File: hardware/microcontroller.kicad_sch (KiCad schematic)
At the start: 12 parts, among them SW1 SW_DPST, U1 ATSAMD21G18A-M, Y1 Crystal

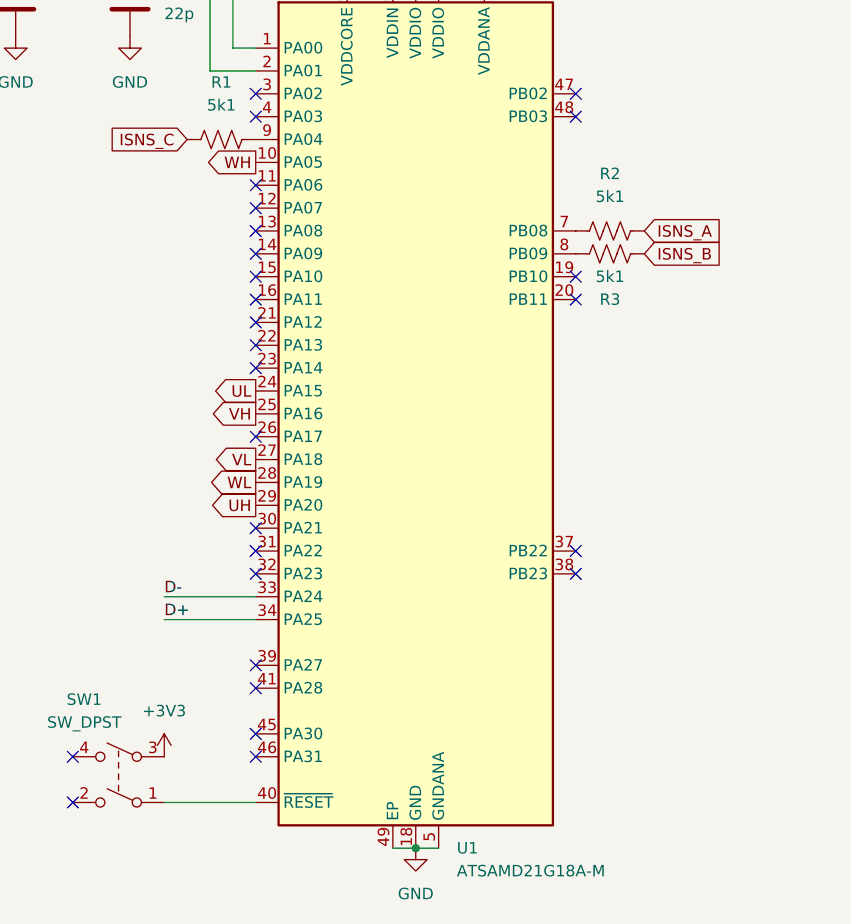
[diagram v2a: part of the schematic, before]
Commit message: Net changes, sense changes
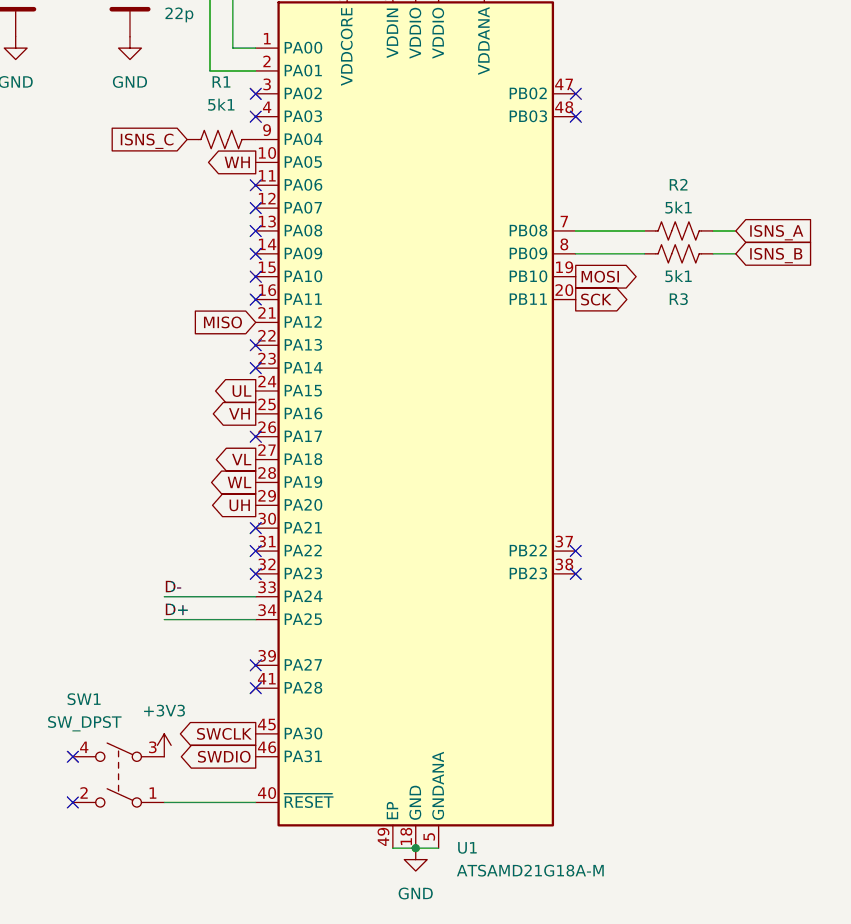
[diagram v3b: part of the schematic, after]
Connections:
- net MOSI: now reaches U1.19 (PB10)
- net SCK: now reaches U1.20 (PB11)
- net MISO: now reaches U1.21 (PA12)
- net SWCLK: now reaches U1.45 (PA30)
- net SWDIO: now reaches U1.46 (PA31)
- no-connect marks 27 -> 22
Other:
- moved on the sheet: R2, R3
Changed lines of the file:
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@@
   (no_connect (at 157.48 116.84))
   (no_connect (at 157.48 119.38))
-  (no_connect (at 157.48 88.9))
-  (no_connect (at 157.48 86.36))
   (no_connect (at 121.92 83.82))
   (no_connect (at 121.92 86.36))
   (no_connect (at 121.92 88.9))
-  (no_connect (at 121.92 91.44))
   (no_connect (at 121.92 93.98))
   (no_connect (at 157.48 66.04))
@@
   (no_connect (at 121.92 114.3))
   (no_connect (at 121.92 104.14))
-  (no_connect (at 121.92 139.7))
-  (no_connect (at 121.92 137.16))
   (no_connect (at 121.92 132.08))
   (no_connect (at 121.92 129.54))
@@
     (stroke (width 0) (type default) (color 0 0 0 0))
   )
+  (wire (pts (xy 165.1 81.28) (xy 157.48 81.28))
+    (stroke (width 0) (type default) (color 0 0 0 0))
+  )
   (wire (pts (xy 105.41 52.07) (xy 107.95 52.07))
     (stroke (width 0) (type default) (color 0 0 0 0))
@@
     (stroke (width 0) (type default) (color 0 0 0 0))
   )
+  (wire (pts (xy 165.1 83.82) (xy 157.48 83.82))
+    (stroke (width 0) (type default) (color 0 0 0 0))
+  )
   (wire (pts (xy 142.24 53.34) (xy 147.32 53.34))
     (stroke (width 0) (type default) (color 0 0 0 0))
@@
   )
   (wire (pts (xy 121.92 63.5) (xy 116.84 63.5))
+    (stroke (width 0) (type default) (color 0 0 0 0))
+  )
+  (wire (pts (xy 175.26 83.82) (xy 172.72 83.82))
+    (stroke (width 0) (type default) (color 0 0 0 0))
+  )
+  (wire (pts (xy 175.26 81.28) (xy 172.72 81.28))
     (stroke (width 0) (type default) (color 0 0 0 0))
   )
@@
     )
   )
+  (global_label "SWDIO" (shape output) (at 121.92 139.7 180) (fields_autoplaced)
+    (effects (font (size 1.27 1.27)) (justify right))
+    (property "Intersheet References" "${INTERSHEET_REFS}" (id 0) (at 113.6407 139.6206 0)
+      (effects (font (size 1.27 1.27)) (justify right) hide)
+    )
+  )
+  (global_label "SWCLK" (shape output) (at 121.92 137.16 180) (fields_autoplaced)
+    (effects (font (size 1.27 1.27)) (justify right))
+    (property "Intersheet References" "${INTERSHEET_REFS}" (id 0) (at 113.2779 137.0806 0)
+      (effects (font (size 1.27 1.27)) (justify right) hide)
+    )
+  )
   (global_label "UL" (shape output) (at 121.92 99.06 180) (fields_autoplaced)
     (effects (font (size 1.27 1.27)) (justify right))
@@
     )
   )
+  (global_label "MISO" (shape input) (at 121.92 91.44 180) (fields_autoplaced)
+    (effects (font (size 1.27 1.27)) (justify right))
+    (property "Intersheet References" "${INTERSHEET_REFS}" (id 0) (at 114.9107 91.3606 0)
+      (effects (font (size 1.27 1.27)) (justify right) hide)
+    )
+  )
   (global_label "ISNS_C" (shape input) (at 114.3 71.12 180) (fields_autoplaced)
     (effects (font (size 1.27 1.27)) (justify right))
@@
     )
   )
-  (global_label "ISNS_A" (shape input) (at 165.1 81.28 0) (fields_autoplaced)
+  (global_label "ISNS_A" (shape input) (at 175.26 81.28 0) (fields_autoplaced)
     (effects (font (size 1.27 1.27)) (justify left))
-    (property "Intersheet References" "${INTERSHEET_REFS}" (id 0) (at 173.9236 81.3594 0)
+    (property "Intersheet References" "${INTERSHEET_REFS}" (id 0) (at 184.0836 81.3594 0)
       (effects (font (size 1.27 1.27)) (justify left) hide)
     )
@@
     )
   )
-  (global_label "ISNS_B" (shape input) (at 165.1 83.82 0) (fields_autoplaced)
+  (global_label "SCK" (shape output) (at 157.48 88.9 0) (fields_autoplaced)
     (effects (font (size 1.27 1.27)) (justify left))
-    (property "Intersheet References" "${INTERSHEET_REFS}" (id 0) (at 174.105 83.8994 0)
+    (property "Intersheet References" "${INTERSHEET_REFS}" (id 0) (at 163.6426 88.8206 0)
+      (effects (font (size 1.27 1.27)) (justify left) hide)
+    )
+  )
+  (global_label "MOSI" (shape output) (at 157.48 86.36 0) (fields_autoplaced)
+    (effects (font (size 1.27 1.27)) (justify left))
+    (property "Intersheet References" "${INTERSHEET_REFS}" (id 0) (at 164.4893 86.2806 0)
+      (effects (font (size 1.27 1.27)) (justify left) hide)
+    )
+  )
+  (global_label "ISNS_B" (shape input) (at 175.26 83.82 0) (fields_autoplaced)
+    (effects (font (size 1.27 1.27)) (justify left))
+    (property "Intersheet References" "${INTERSHEET_REFS}" (id 0) (at 184.265 83.8994 0)
       (effects (font (size 1.27 1.27)) (justify left) hide)
     )
@@
     (pin "2")
   )
-  (symbol (lib_id "Device:R_US") (at 161.29 83.82 90) (unit 1)
+  (symbol (lib_id "Device:R_US") (at 168.91 83.82 90) (unit 1)
     (in_bom yes) (on_board yes)
-    (property "Reference" "R3" (id 0) (at 161.29 88.9 90))
-    (property "Value" "5k1" (id 1) (at 161.29 86.36 90))
-    (property "Footprint" "Resistor_SMD:R_0805_2012Metric" (id 2) (at 161.544 82.804 90)
-      (effects (font (size 1.27 1.27)) hide)
-    )
-    (property "Datasheet" "~" (id 3) (at 161.29 83.82 0)
-      (effects (font (size 1.27 1.27)) hide)
-    )
-    (property "Mouser" "https://www.mouser.com/ProductDetail/Panasonic/ERJ-6ENF5101V?qs=sGAEpiMZZMvdGkrng054t8AJgcdMkx7xVxAUQLZTFHA%3D" (id 4) (at 161.29 83.82 90)
+    (property "Reference" "R3" (id 0) (at 168.91 88.9 90))
+    (property "Value" "5k1" (id 1) (at 168.91 86.36 90))
+    (property "Footprint" "Resistor_SMD:R_0805_2012Metric" (id 2) (at 169.164 82.804 90)
+      (effects (font (size 1.27 1.27)) hide)
+    )
+    (property "Datasheet" "~" (id 3) (at 168.91 83.82 0)
+      (effects (font (size 1.27 1.27)) hide)
+    )
+    (property "Mouser" "https://www.mouser.com/ProductDetail/Panasonic/ERJ-6ENF5101V?qs=sGAEpiMZZMvdGkrng054t8AJgcdMkx7xVxAUQLZTFHA%3D" (id 4) (at 168.91 83.82 90)
       (effects (font (size 1.27 1.27)) hide)
     )
@@
     (pin "2")
   )
-  (symbol (lib_id "Device:R_US") (at 161.29 81.28 90) (unit 1)
-    (in_bom yes) (on_board yes) (fields_autoplaced)
-    (property "Reference" "R2" (id 0) (at 161.29 74.93 90))
-    (property "Value" "5k1" (id 1) (at 161.29 77.47 90))
-    (property "Footprint" "Resistor_SMD:R_0805_2012Metric" (id 2) (at 161.544 80.264 90)
-      (effects (font (size 1.27 1.27)) hide)
-    )
-    (property "Datasheet" "~" (id 3) (at 161.29 81.28 0)
-      (effects (font (size 1.27 1.27)) hide)
-    )
-    (property "Mouser" "https://www.mouser.com/ProductDetail/Panasonic/ERJ-6ENF5101V?qs=sGAEpiMZZMvdGkrng054t8AJgcdMkx7xVxAUQLZTFHA%3D" (id 4) (at 161.29 81.28 90)
-      (effects (font (size 1.27 1.27)) hide)
-    )
+  (symbol (lib_id "Device:R_US") (at 168.91 81.28 90) (unit 1)
+    (in_bom yes) (on_board yes)
+    (property "Reference" "R2" (id 0) (at 168.91 76.2 90))
+    (property "Value" "5k1" (id 1) (at 168.91 78.74 90))
+    (property "Footprint" "Resistor_SMD:R_0805_2012Metric" (id 2) (at 169.164 80.264 90)
+      (effects (font (size 1.27 1.27)) hide)
+    )
+    (property "Datasheet" "~" (id 3) (at 168.91 81.28 0)
+      (effects (font (size 1.27 1.27)) hide)
+    )
+    (property "Mouser" "https://www.mouser.com/ProductDetail/Panasonic/ERJ-6ENF5101V?qs=sGAEpiMZZMvdGkrng054t8AJgcdMkx7xVxAUQLZTFHA%3D" (id 4) (at 168.91 81.28 90)
+      (effects (font (size 1.27 1.27)) hide)
+    )

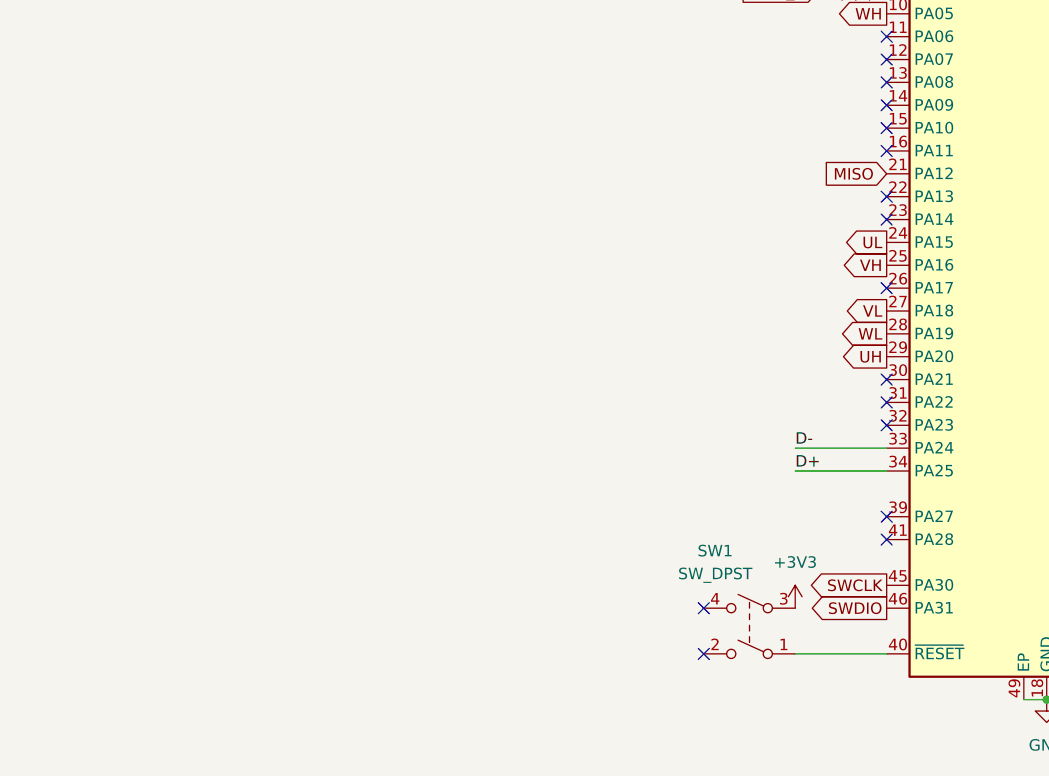
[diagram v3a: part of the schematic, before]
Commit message: swd interface
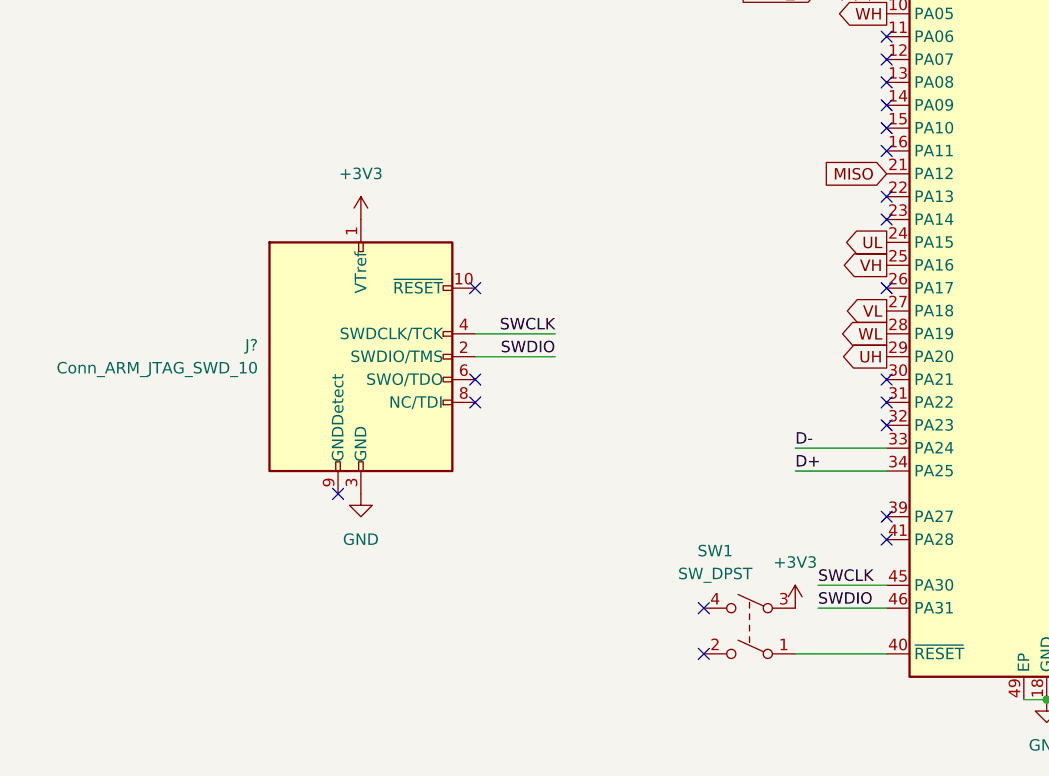
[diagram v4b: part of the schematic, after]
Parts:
- added J?: Conn_ARM_JTAG_SWD_10, Connector_PinHeader_1.27mm:PinHeader_2x05_P1.27mm_Vertical_SMD, symbol Connector:Conn_ARM_JTAG_SWD_10
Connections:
- net +3V3: now also J?.1 (VTref)
- net GND: now also J?.3 (GND), J?.5 (GND)
- net SWCLK: now also J?.4 (SWDCLK/TCK)
- net SWDIO: now also J?.2 (SWDIO/TMS)
- no-connect marks 22 -> 26
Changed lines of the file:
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@@
   (junction (at 95.25 52.07) (diameter 0) (color 0 0 0 0)
   )
+  (no_connect (at 60.96 127))
   (no_connect (at 121.92 66.04))
   (no_connect (at 121.92 68.58))
@@
   (no_connect (at 121.92 132.08))
   (no_connect (at 121.92 129.54))
+  (no_connect (at 76.2 104.14))
+  (no_connect (at 76.2 114.3))
+  (no_connect (at 76.2 116.84))
   (wire (pts (xy 132.08 31.75) (xy 143.51 31.75))
     (stroke (width 0) (type default) (color 0 0 0 0))
@@
     (stroke (width 0) (type default) (color 0 0 0 0))
   )
+  (wire (pts (xy 114.3 139.7) (xy 121.92 139.7))
+    (stroke (width 0) (type default) (color 0 0 0 0))
+  )
   (wire (pts (xy 175.26 83.82) (xy 172.72 83.82))
     (stroke (width 0) (type default) (color 0 0 0 0))
   )
+  (wire (pts (xy 114.3 137.16) (xy 121.92 137.16))
+    (stroke (width 0) (type default) (color 0 0 0 0))
+  )
+  (wire (pts (xy 76.2 111.76) (xy 85.09 111.76))
+    (stroke (width 0) (type default) (color 0 0 0 0))
+  )
   (wire (pts (xy 175.26 81.28) (xy 172.72 81.28))
     (stroke (width 0) (type default) (color 0 0 0 0))
@@
     (stroke (width 0) (type default) (color 0 0 0 0))
   )
+  (wire (pts (xy 76.2 109.22) (xy 85.09 109.22))
+    (stroke (width 0) (type default) (color 0 0 0 0))
+  )
   (wire (pts (xy 116.84 63.5) (xy 116.84 52.07))
     (stroke (width 0) (type default) (color 0 0 0 0))
@@
     (effects (font (size 1.27 1.27)) (justify left bottom))
   )
+  (label "SWDIO" (at 114.3 139.7 0)
+    (effects (font (size 1.27 1.27)) (justify left bottom))
+  )
+  (label "SWCLK" (at 85.09 109.22 180)
+    (effects (font (size 1.27 1.27)) (justify right bottom))
+  )
+  (label "SWDIO" (at 85.09 111.76 180)
+    (effects (font (size 1.27 1.27)) (justify right bottom))
+  )
   (label "D-" (at 111.76 121.92 0)
     (effects (font (size 1.27 1.27)) (justify left bottom))
@@
     (effects (font (size 1.27 1.27)) (justify left bottom))
   )
+  (label "SWCLK" (at 114.3 137.16 0)
+    (effects (font (size 1.27 1.27)) (justify left bottom))
+  )
   (global_label "VL" (shape output) (at 121.92 106.68 180) (fields_autoplaced)
     (effects (font (size 1.27 1.27)) (justify right))
@@
     (effects (font (size 1.27 1.27)) (justify right))
     (property "Intersheet References" "${INTERSHEET_REFS}" (id 0) (at 117.0274 109.1406 0)
-      (effects (font (size 1.27 1.27)) (justify right) hide)
-    )
-  )
-  (global_label "SWDIO" (shape output) (at 121.92 139.7 180) (fields_autoplaced)
-    (effects (font (size 1.27 1.27)) (justify right))
-    (property "Intersheet References" "${INTERSHEET_REFS}" (id 0) (at 113.6407 139.6206 0)
-      (effects (font (size 1.27 1.27)) (justify right) hide)
-    )
-  )
-  (global_label "SWCLK" (shape output) (at 121.92 137.16 180) (fields_autoplaced)
-    (effects (font (size 1.27 1.27)) (justify right))
-    (property "Intersheet References" "${INTERSHEET_REFS}" (id 0) (at 113.2779 137.0806 0)
       (effects (font (size 1.27 1.27)) (justify right) hide)
     )
@@
     (pin "2")
   )
+  (symbol (lib_id "Connector:Conn_ARM_JTAG_SWD_10") (at 63.5 111.76 0) (unit 1)
+    (in_bom yes) (on_board yes) (fields_autoplaced)
+    (property "Reference" "J?" (id 0) (at 52.07 110.4899 0)
+      (effects (font (size 1.27 1.27)) (justify right))
+    )
+    (property "Value" "Conn_ARM_JTAG_SWD_10" (id 1) (at 52.07 113.0299 0)
+      (effects (font (size 1.27 1.27)) (justify right))
+    )
+    (property "Footprint" "Connector_PinHeader_1.27mm:PinHeader_2x05_P1.27mm_Vertical_SMD" (id 2) (at 63.5 111.76 0)
+      (effects (font (size 1.27 1.27)) hide)
+    )
+    (property "Datasheet" "http://infocenter.arm.com/help/topic/com.arm.doc.ddi0314h/DDI0314H_coresight_components_trm.pdf" (id 3) (at 54.61 143.51 90)
+      (effects (font (size 1.27 1.27)) hide)
+    )
+    (pin "1")
+    (pin "10")
+    (pin "2")
+    (pin "3")
+    (pin "4")
+    (pin "5")
+    (pin "6")
+    (pin "7")
+    (pin "8")
+    (pin "9")
+  )
   (symbol (lib_id "power:GND") (at 107.95 59.69 0) (unit 1)
     (in_bom yes) (on_board yes) (fields_autoplaced)
@@
     (pin "2")
   )
+  (symbol (lib_id "power:GND") (at 63.5 127 0) (unit 1)
+    (in_bom yes) (on_board yes) (fields_autoplaced)
+    (property "Reference" "#PWR?" (id 0) (at 63.5 133.35 0)
+      (effects (font (size 1.27 1.27)) hide)
+    )
+    (property "Value" "GND" (id 1) (at 63.5 132.08 0))
+    (property "Footprint" "" (id 2) (at 63.5 127 0)
+      (effects (font (size 1.27 1.27)) hide)
+    )
+    (property "Datasheet" "" (id 3) (at 63.5 127 0)
+      (effects (font (size 1.27 1.27)) hide)
+    )
+    (pin "1")
+  )
   (symbol (lib_id "power:GND") (at 95.25 59.69 0) (unit 1)
     (in_bom yes) (on_board yes) (fields_autoplaced)
@@
     (pin "2")
   )
+  (symbol (lib_id "power:+3V3") (at 63.5 96.52 0) (unit 1)
+    (in_bom yes) (on_board yes) (fields_autoplaced)
+    (property "Reference" "#PWR?" (id 0) (at 63.5 100.33 0)
+      (effects (font (size 1.27 1.27)) hide)
+    )
+    (property "Value" "+3V3" (id 1) (at 63.5 91.44 0))
+    (property "Footprint" "" (id 2) (at 63.5 96.52 0)
+      (effects (font (size 1.27 1.27)) hide)
+    )
+    (property "Datasheet" "" (id 3) (at 63.5 96.52 0)
+      (effects (font (size 1.27 1.27)) hide)
+    )
+    (pin "1")
+  )
   (symbol (lib_id "power:+3V3") (at 111.76 139.7 0) (unit 1)
